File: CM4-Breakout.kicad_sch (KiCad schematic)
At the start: 2 parts

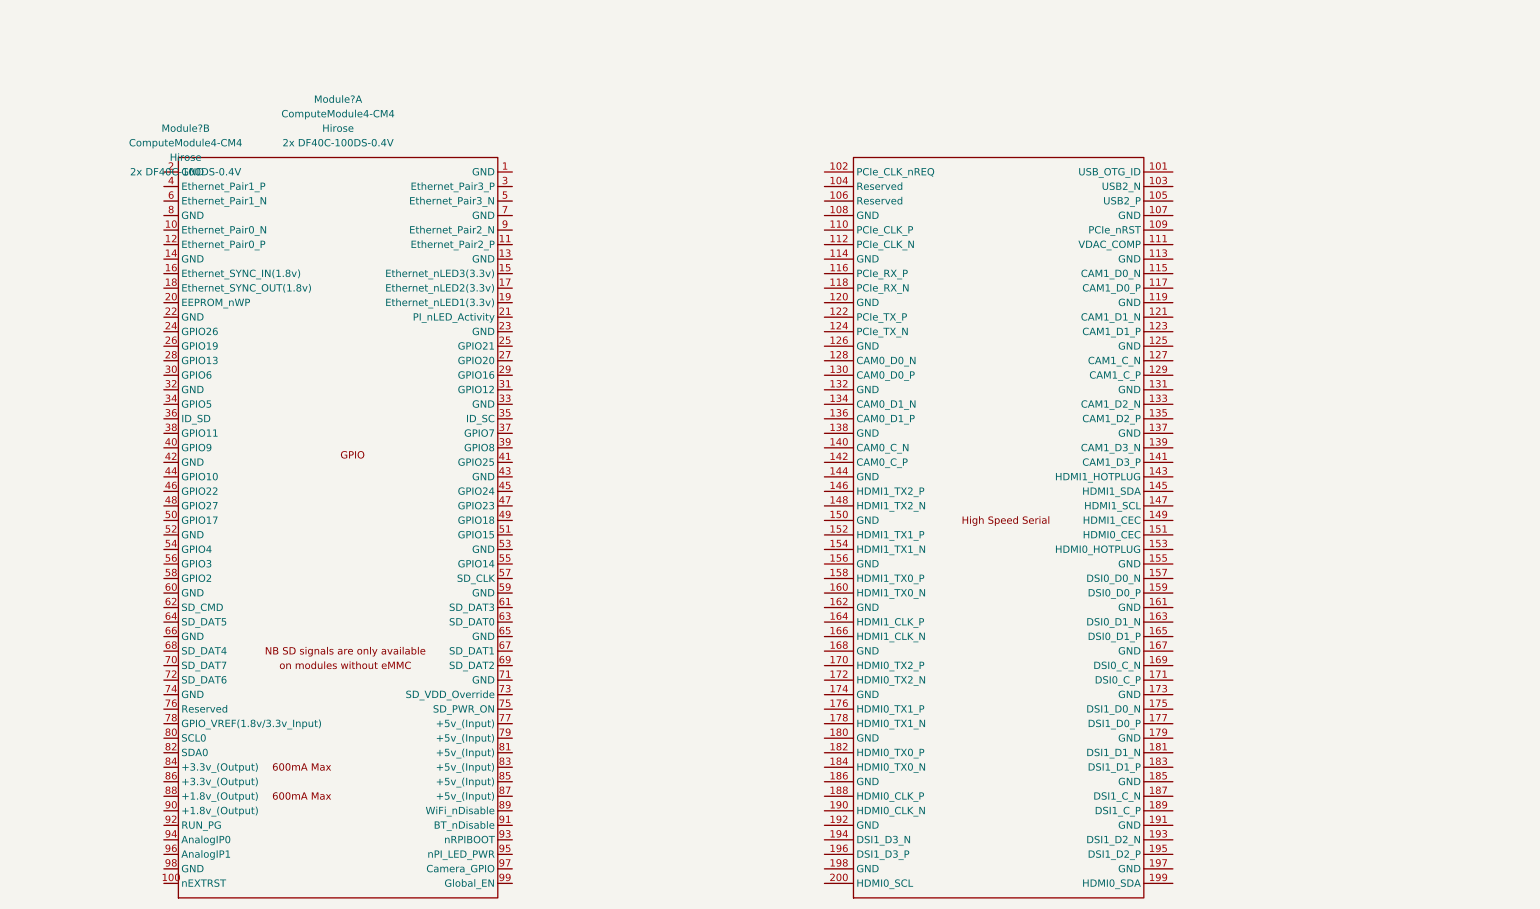
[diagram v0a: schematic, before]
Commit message: Some work was done
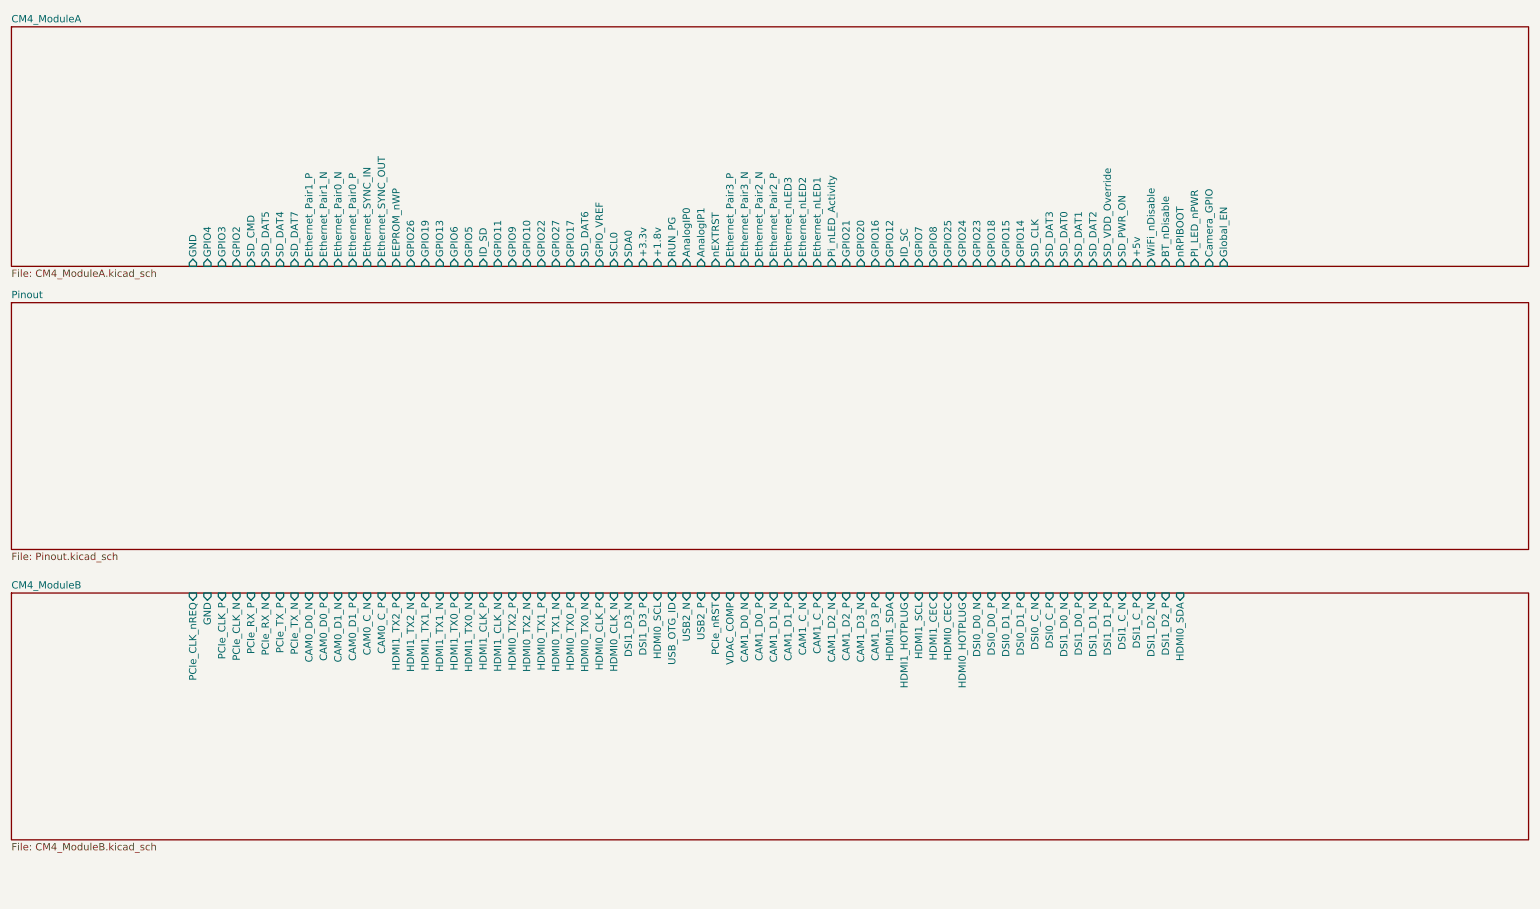
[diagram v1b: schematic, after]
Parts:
- removed Module? (x2): ComputeModule4-CM4, CM4IO:Raspberry-Pi-4-Compute-Module, symbol CM4IO:ComputeModule4-CM4
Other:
- added sheet CM4_ModuleA (CM4_ModuleA.kicad_sch)
- added sheet CM4_ModuleB (CM4_ModuleB.kicad_sch)
- added sheet Pinout (Pinout.kicad_sch)
